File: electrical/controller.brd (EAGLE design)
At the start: 101.6 x 25.4 mm, 36 parts, among them IC1 MCP6232, IC2 LTC1661MSOP8, IC3 MCP6232, IC4 ICM7555, IC5 CD40109B, J3 455-1750-1-ND, Q1 DMP3098, Q3 600mA/40V, U1 U3V16F15, U2 U3V16F15

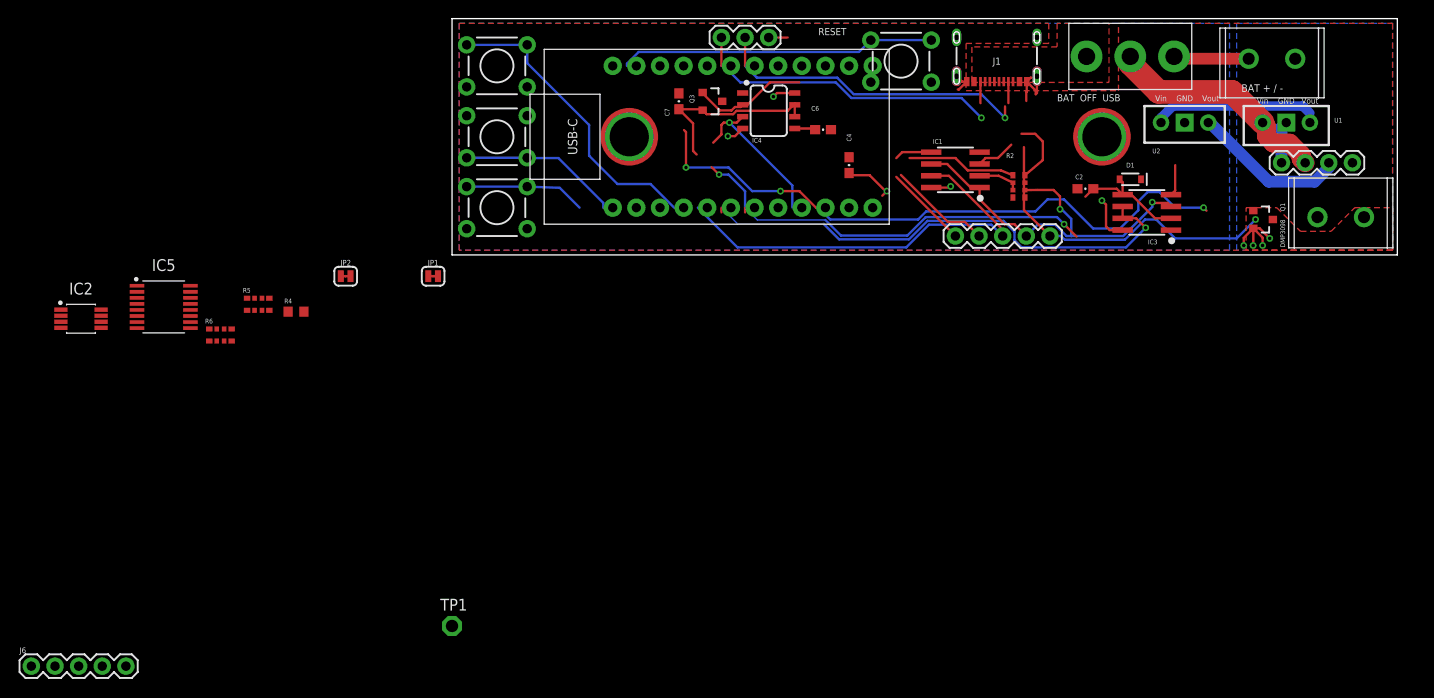
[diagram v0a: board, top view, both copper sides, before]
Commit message: Plop some things onto the PCB, lots of work to do.
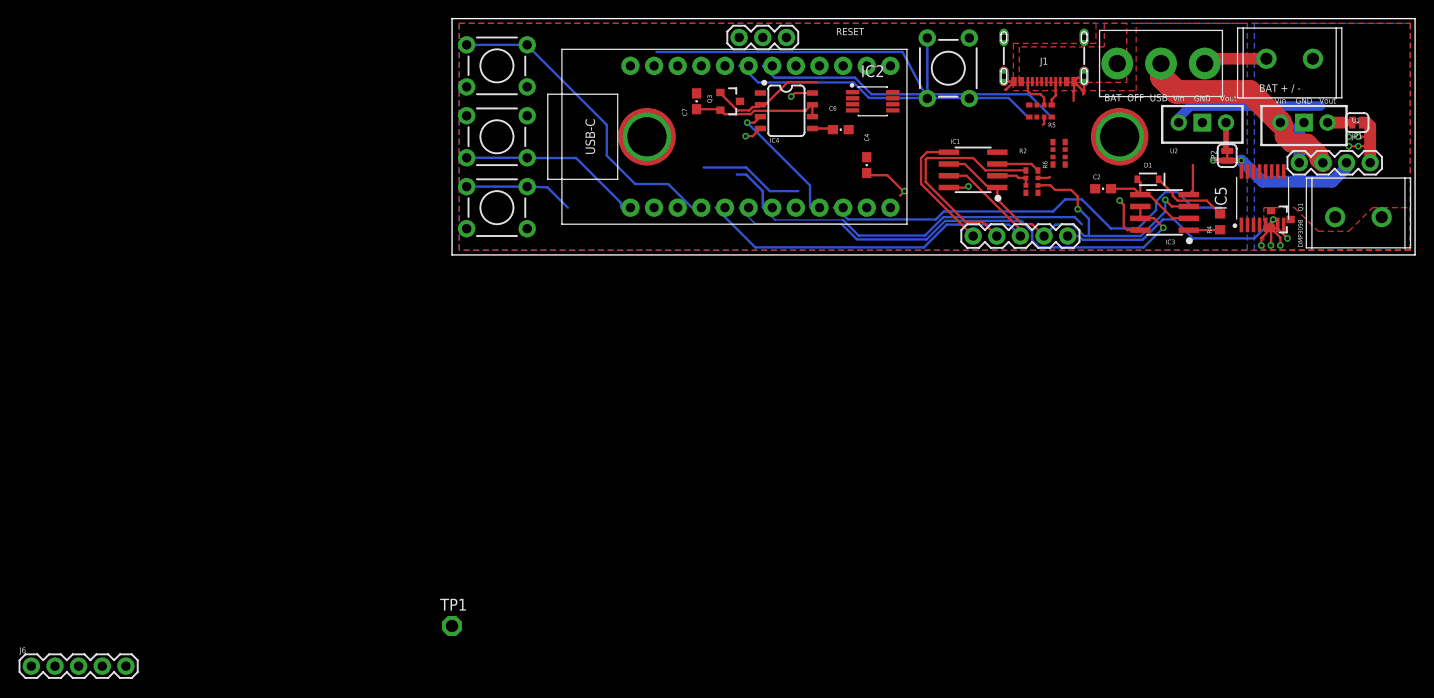
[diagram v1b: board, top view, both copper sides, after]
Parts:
- moved IC5 118.7 mm to (87.1, 6.10), turned to 90 degrees
- moved JP1 100.7 mm to (97.3, 14.2), turned to 180 degrees
- moved R4 99.8 mm to (82.5, 3.56), turned to 90 degrees
- moved JP2 95.6 mm to (83.3, 10.7), turned to 90 degrees
- moved R6 92.3 mm to (65.3, 10.9), turned to 90 degrees
- moved IC2 88.2 mm to (45.2, 16.5)
- moved R5 86.6 mm to (63.2, 15.5), turned to 180 degrees
- moved S4 5.14 mm to (53.3, 20.1), turned to 270 degrees
- moved J1 5.08 mm to (63.6, 18.3)
- moved S_PWR 3.39 mm to (76.2, 20.6)
- moved C2 1.91 mm to (70.0, 7.11)
- moved C4 1.91 mm to (44.6, 9.65)
- moved C6 1.91 mm to (41.8, 13.5)
- moved C7 1.91 mm to (26.3, 16.5)
- moved D1 1.91 mm to (74.8, 8.13)
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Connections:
- removed net 12V: IC5.16, JP1.1
- net 15V: now also IC5.16, JP1.1
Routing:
- net COIL: track 35.6 -> 24.9 mm
- net DRIVE: track 67.6 -> 58.5 mm, vias 3 -> 0
- net 15V: track 26.1 -> 34.6 mm, vias 4 -> 8
- net N$1: track 0.00 -> 8.29 mm
- net N$4: track 11.4 -> 4.66 mm
- net N$7: track 20.2 -> 14.5 mm
- net PEAK_RST: track 58.2 -> 53.4 mm, vias 2 -> 0
- net RST: track 34.0 -> 38.6 mm
- net N$2: track 0.00 -> 3.39 mm
- net TIMER_RESTART: track 16.9 -> 13.6 mm
- net N$9: track 0.00 -> 3.09 mm
- net N$8: track 0.00 -> 2.65 mm
- net GND: track 17.9 -> 20.1 mm
- net TIMER_RST: track 14.5 -> 12.5 mm
- net USR2: track 17.2 -> 19.1 mm
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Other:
- board size 101.6 x 25.4 mm -> 103.5 x 25.4 mm
